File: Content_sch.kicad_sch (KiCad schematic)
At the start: 0 parts

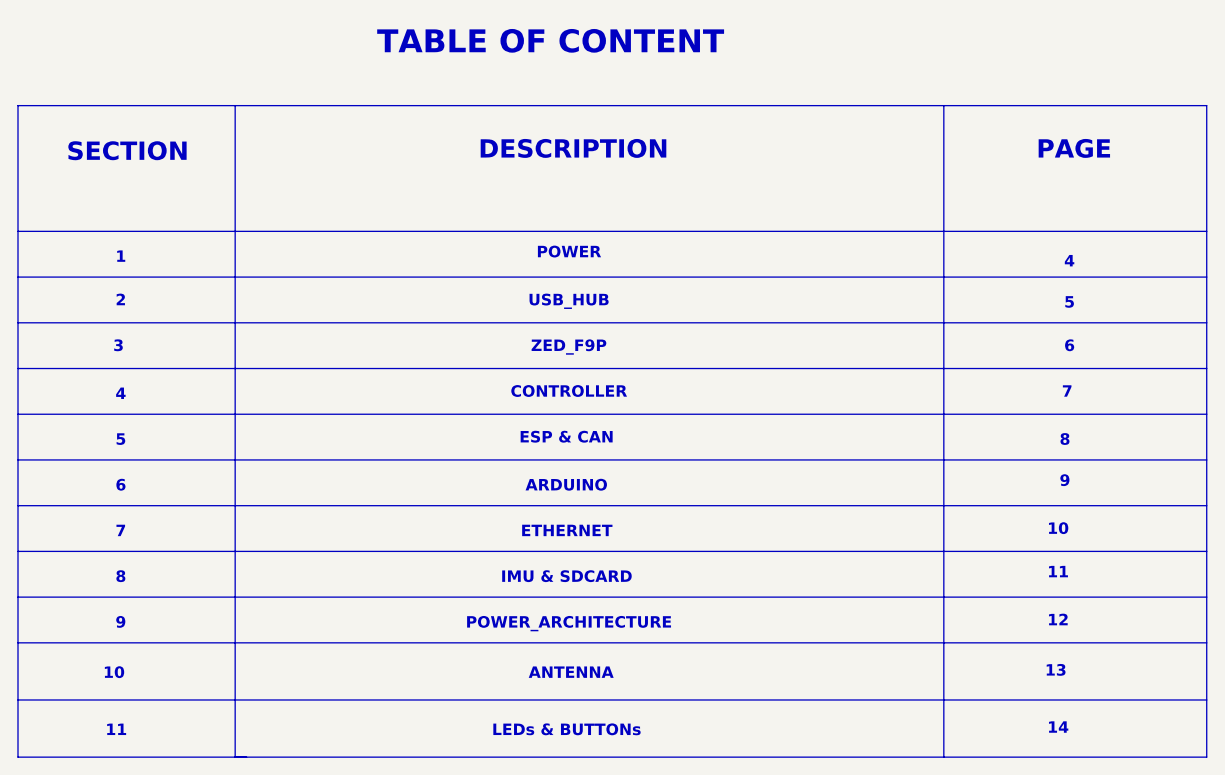
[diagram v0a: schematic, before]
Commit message: 18.09.2026
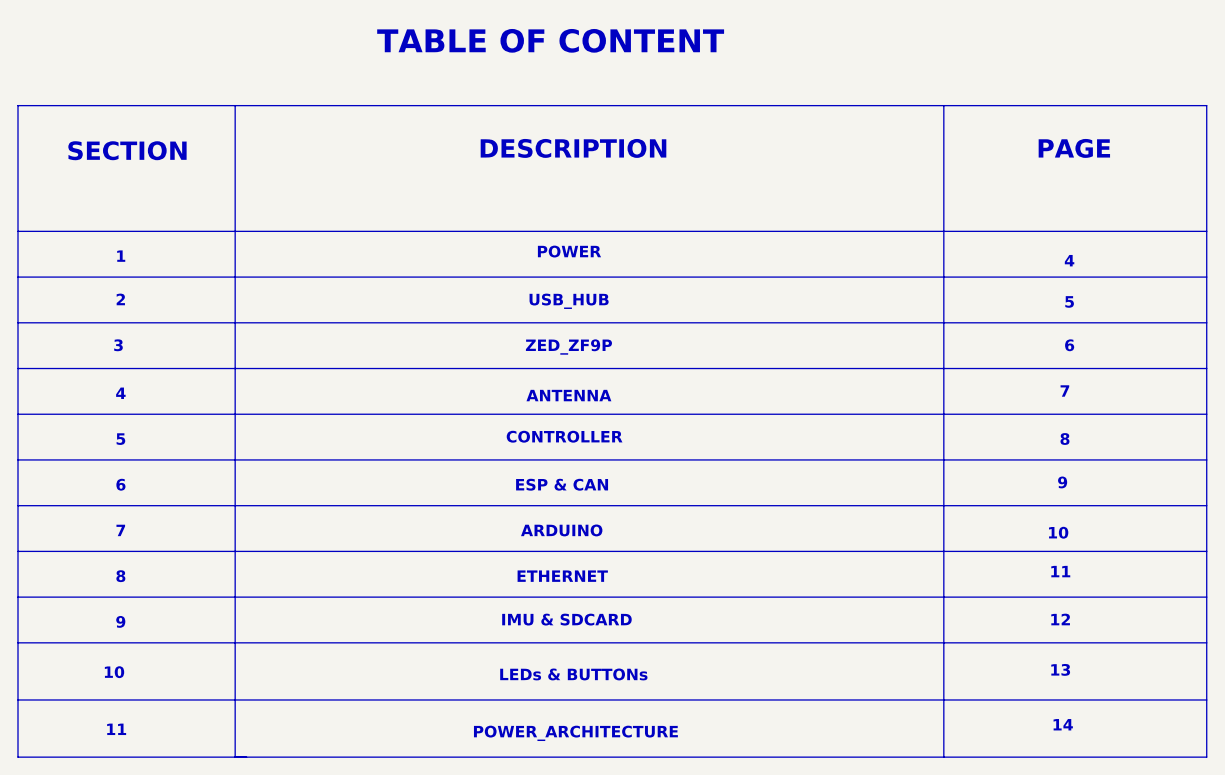
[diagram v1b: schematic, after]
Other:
- note added: "ZED_ZF9P"
- note removed: "ZED_F9P"
